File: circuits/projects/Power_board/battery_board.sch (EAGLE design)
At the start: 30 parts

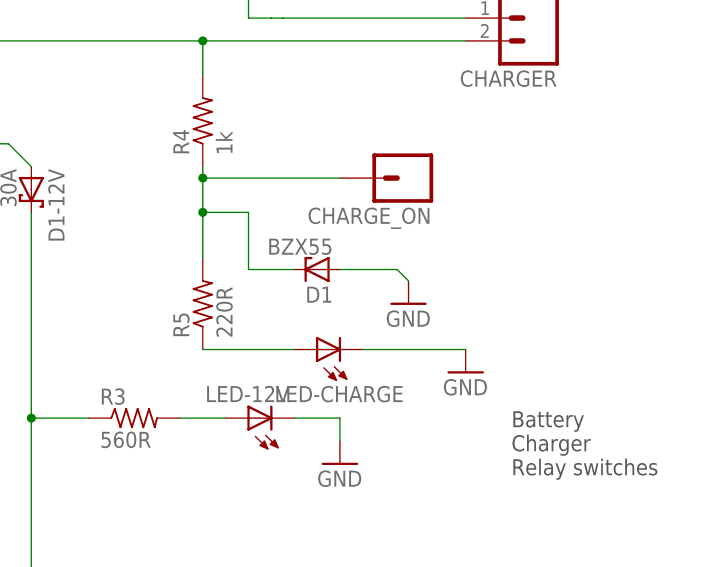
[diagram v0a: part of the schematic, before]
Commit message: fixed board error
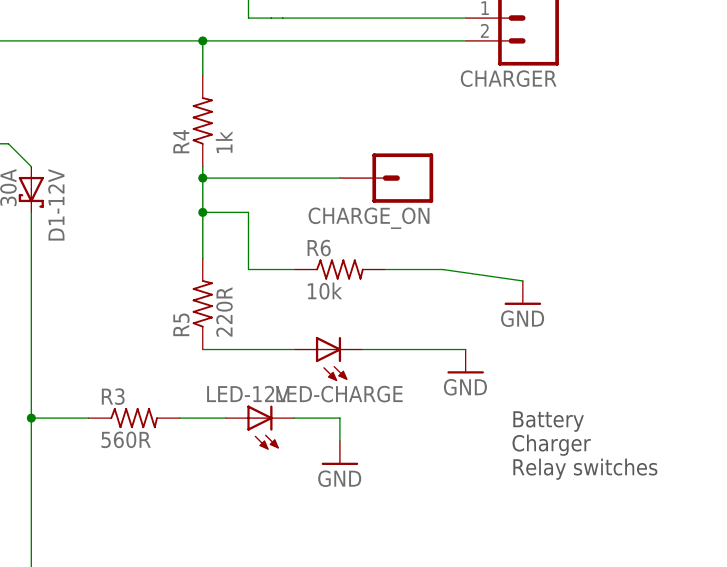
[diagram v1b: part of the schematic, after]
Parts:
- removed D1: BZX55, parts:BZX55
- added R6: 10k, parts:RESISTOR0207/10
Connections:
- net GND: no longer D1.A
- net N$15: now also R6.1; no longer D1.C
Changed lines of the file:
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@@
 <setting verticaltext="up"/>
 </settings>
-<grid distance="0.05" unitdist="inch" unit="inch" style="lines" multiple="1" display="yes" altdistance="0.025" altunitdist="inch" altunit="inch"/>
+<grid distance="0.1" unitdist="inch" unit="inch" style="lines" multiple="1" display="no" altdistance="0.01" altunitdist="inch" altunit="inch"/>
 <layers>
 <layer number="1" name="Top" color="4" fill="1" visible="no" active="no"/>
@@
 <part name="FUSE-M2" library="parts" deviceset="2-HOLES" device="SC5MM" value="3A"/>
 <part name="FUSE-M1" library="parts" deviceset="2-HOLES" device="SC5MM" value="3A"/>
-<part name="D1" library="parts" deviceset="BZX55" device=""/>
 <part name="GND7" library="parts" deviceset="GND" device=""/>
+<part name="R6" library="parts" deviceset="RESISTOR" device="0207/10" value="10k"/>
 </parts>
 <sheets>
@@
 <instance part="FUSE-M2" gate="G$1" x="20.32" y="63.5" rot="R180"/>
 <instance part="FUSE-M1" gate="G$1" x="41.91" y="63.5" rot="R180"/>
-<instance part="D1" gate="1" x="172.72" y="44.45" rot="R180"/>
-<instance part="GND7" gate="1" x="182.88" y="40.64"/>
+<instance part="GND7" gate="1" x="195.58" y="40.64"/>
+<instance part="R6" gate="G$1" x="175.26" y="44.45"/>
 </instances>
 <busses>
@@
 <segment>
 <pinref part="GND7" gate="1" pin="GND"/>
-<pinref part="D1" gate="1" pin="A"/>
-<wire x1="182.88" y1="43.18" x2="181.61" y2="44.45" width="0.1524" layer="91"/>
-<wire x1="181.61" y1="44.45" x2="175.26" y2="44.45" width="0.1524" layer="91"/>
+<wire x1="195.58" y1="43.18" x2="186.69" y2="44.45" width="0.1524" layer="91"/>
+<wire x1="186.69" y1="44.45" x2="180.34" y2="44.45" width="0.1524" layer="91"/>
 </segment>
 </net>
@@
 <wire x1="175.26" y1="54.61" x2="160.02" y2="54.61" width="0.1524" layer="91"/>
 <junction x="160.02" y="54.61"/>
-<pinref part="D1" gate="1" pin="C"/>
 <wire x1="170.18" y1="44.45" x2="165.1" y2="44.45" width="0.1524" layer="91"/>
 <wire x1="165.1" y1="44.45" x2="165.1" y2="50.8" width="0.1524" layer="91"/>
 <wire x1="165.1" y1="50.8" x2="160.02" y2="50.8" width="0.1524" layer="91"/>
 <junction x="160.02" y="50.8"/>
-</segment>
-</net>
+<pinref part="R6" gate="G$1" pin="1"/>
+</segment>
+</net>

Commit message: Revert "fixed board error"
This reverts commit a9d72898da9c7dfbc8182aee948ad086d6644fb1.
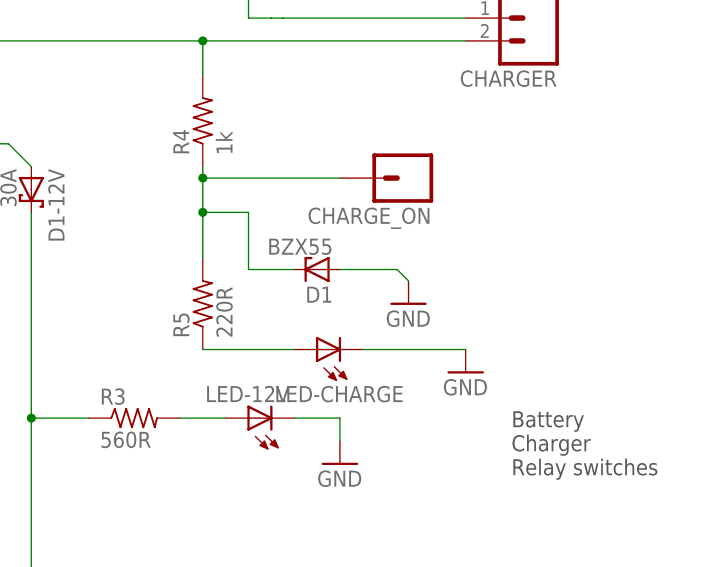
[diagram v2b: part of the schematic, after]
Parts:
- removed R6: 10k, parts:RESISTOR0207/10
- added D1: BZX55, parts:BZX55
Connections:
- net GND: now also D1.A
- net N$15: now also D1.C; no longer R6.1
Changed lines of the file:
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@@
 <setting verticaltext="up"/>
 </settings>
-<grid distance="0.1" unitdist="inch" unit="inch" style="lines" multiple="1" display="no" altdistance="0.01" altunitdist="inch" altunit="inch"/>
+<grid distance="0.05" unitdist="inch" unit="inch" style="lines" multiple="1" display="yes" altdistance="0.025" altunitdist="inch" altunit="inch"/>
 <layers>
 <layer number="1" name="Top" color="4" fill="1" visible="no" active="no"/>
@@
 <part name="FUSE-M2" library="parts" deviceset="2-HOLES" device="SC5MM" value="3A"/>
 <part name="FUSE-M1" library="parts" deviceset="2-HOLES" device="SC5MM" value="3A"/>
+<part name="D1" library="parts" deviceset="BZX55" device=""/>
 <part name="GND7" library="parts" deviceset="GND" device=""/>
-<part name="R6" library="parts" deviceset="RESISTOR" device="0207/10" value="10k"/>
 </parts>
 <sheets>
@@
 <instance part="FUSE-M2" gate="G$1" x="20.32" y="63.5" rot="R180"/>
 <instance part="FUSE-M1" gate="G$1" x="41.91" y="63.5" rot="R180"/>
-<instance part="GND7" gate="1" x="195.58" y="40.64"/>
-<instance part="R6" gate="G$1" x="175.26" y="44.45"/>
+<instance part="D1" gate="1" x="172.72" y="44.45" rot="R180"/>
+<instance part="GND7" gate="1" x="182.88" y="40.64"/>
 </instances>
 <busses>
@@
 <segment>
 <pinref part="GND7" gate="1" pin="GND"/>
-<wire x1="195.58" y1="43.18" x2="186.69" y2="44.45" width="0.1524" layer="91"/>
-<wire x1="186.69" y1="44.45" x2="180.34" y2="44.45" width="0.1524" layer="91"/>
+<pinref part="D1" gate="1" pin="A"/>
+<wire x1="182.88" y1="43.18" x2="181.61" y2="44.45" width="0.1524" layer="91"/>
+<wire x1="181.61" y1="44.45" x2="175.26" y2="44.45" width="0.1524" layer="91"/>
 </segment>
 </net>
@@
 <wire x1="175.26" y1="54.61" x2="160.02" y2="54.61" width="0.1524" layer="91"/>
 <junction x="160.02" y="54.61"/>
+<pinref part="D1" gate="1" pin="C"/>
 <wire x1="170.18" y1="44.45" x2="165.1" y2="44.45" width="0.1524" layer="91"/>
 <wire x1="165.1" y1="44.45" x2="165.1" y2="50.8" width="0.1524" layer="91"/>
 <wire x1="165.1" y1="50.8" x2="160.02" y2="50.8" width="0.1524" layer="91"/>
 <junction x="160.02" y="50.8"/>
-<pinref part="R6" gate="G$1" pin="1"/>
-</segment>
-</net>
+</segment>
+</net>
